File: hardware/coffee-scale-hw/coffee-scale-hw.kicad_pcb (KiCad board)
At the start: 2 copper layers, 60 x 35 mm, 63 parts, among them J1 PWR_IN, J2 OLED, J3 LOAD_CELL, Q1 AO3401A, Q2 AO3401A, Q3 PNP, SW1 SW_SPDT, SW2 SW_BACK, SW3 SW_L, SW4 SW_R, SW5 SW_OK, U1 TLV61046ADB, U2 STM32F103C8Tx, U3 HX711

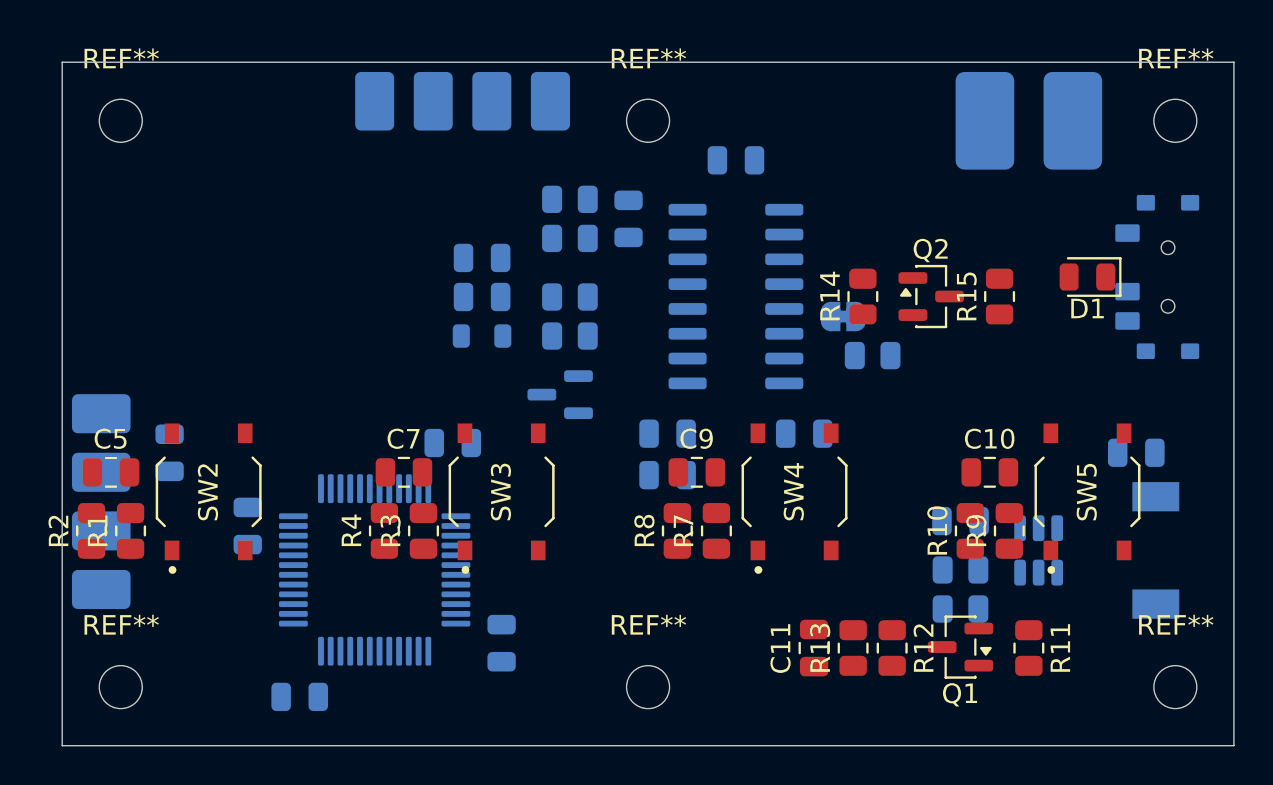
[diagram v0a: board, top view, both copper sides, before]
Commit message: Working on HW design
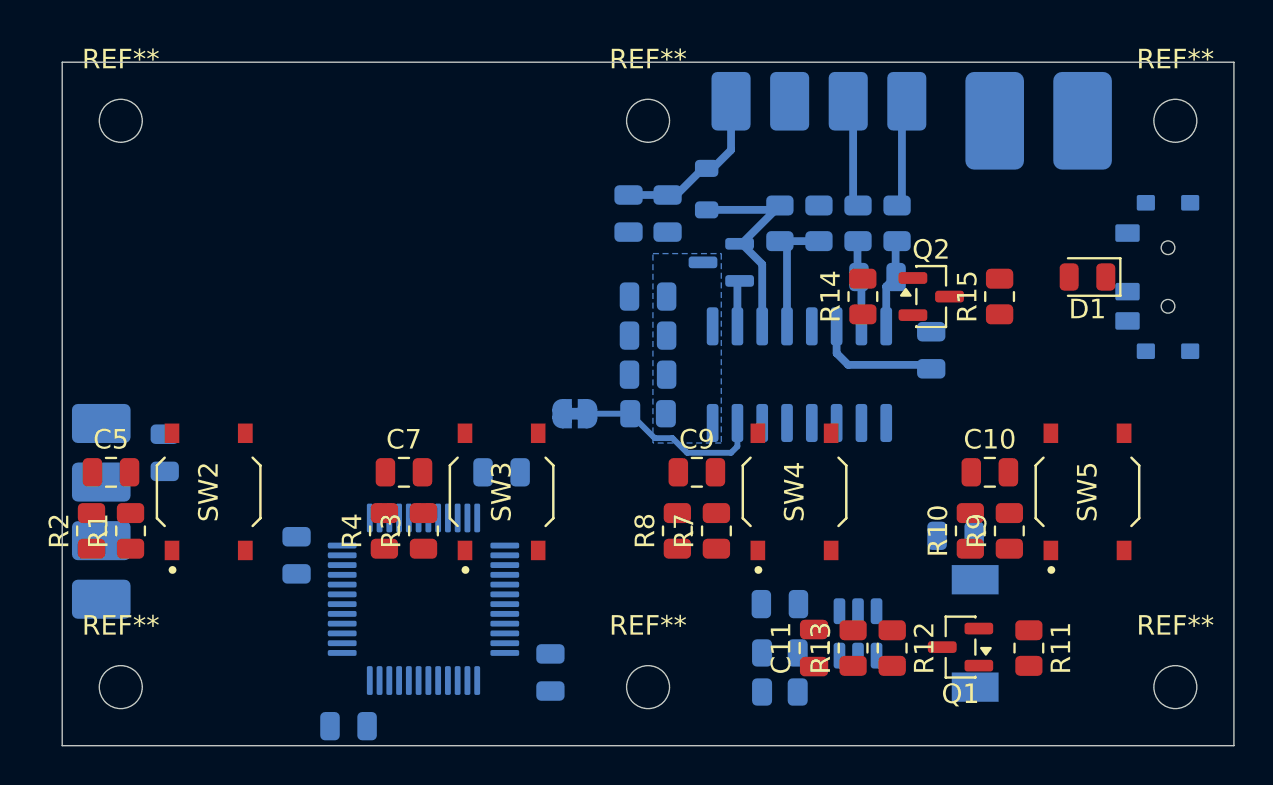
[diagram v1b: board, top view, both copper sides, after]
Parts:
- moved J3 18.2 mm to (168.8, 80.0)
- moved R18 16.8 mm to (172.8, 88.2), turned to 90 degrees
- moved R19 14.8 mm to (170.8, 88.2), turned to 90 degrees
- moved JP1 14.6 mm to (156.2, 98.0)
- moved C17 14.0 mm to (174.5, 94.8), turned to 90 degrees
- moved L2 13.7 mm to (163.0, 86.5), turned to -90 degrees
- moved R16 13.3 mm to (168.8, 88.2), turned to 90 degrees
- moved C14 13.1 mm to (171.8, 91.0), turned to 180 degrees
- moved R17 12.2 mm to (166.8, 88.2), turned to -90 degrees
- moved R20 11.9 mm to (160.0, 98.0)
- moved Q3 10.7 mm to (163.8, 90.2)
- moved C6 10.2 mm to (175.8, 104.2)
- moved C8 10.2 mm to (166.8, 107.8)
- moved L1 10.2 mm to (176.8, 109.2)
- moved R5 10.2 mm to (166.8, 110.2)
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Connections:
- J1 pad 1: Net-(J1-Pin_1) -> GND
- J1 pad 2: GND -> Net-(J1-Pin_2)
- SW1 pad 2: Net-(J1-Pin_1) -> Net-(J1-Pin_2)
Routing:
- net Net-(Q3-C): track 0.00 -> 11.5 mm
- net Net-(JP1-A): track 0.00 -> 9.84 mm
- net HX711_E+: track 0.00 -> 8.70 mm
- net Net-(U3-VBG): track 0.00 -> 6.55 mm
- net Net-(U3-VFB): track 0.00 -> 6.51 mm
- net HX711_A-: track 0.00 -> 5.54 mm
- net HX711_A+: track 0.00 -> 5.54 mm
- net Net-(U3-INA+): track 0.00 -> 4.63 mm
- net Net-(U3-INA-): track 0.00 -> 4.45 mm
- net Net-(Q3-B): track 0.00 -> 2.37 mm
- added copper zone on B.Cu, net +5V
